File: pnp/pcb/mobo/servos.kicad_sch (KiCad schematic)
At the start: 2 parts, among them J15 SERVO1, J16 SERVO2

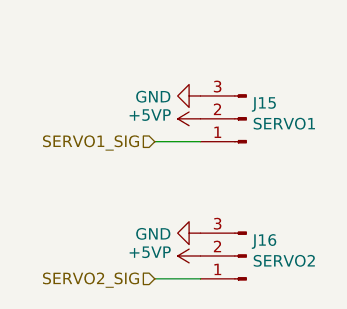
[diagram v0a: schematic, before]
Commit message: All sheets cleaned up
All symbols and their fields are now neatly organized.

All hierarchical pins are already imported,
except for the microcontroller sheet.
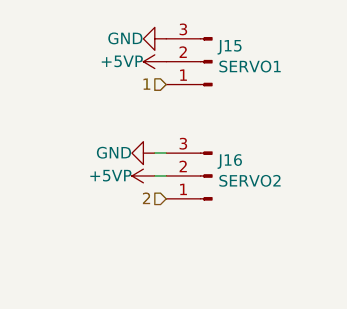
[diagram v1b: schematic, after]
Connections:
- net SERVO1_SIG renamed 1
- net SERVO2_SIG renamed 2
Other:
- moved on the sheet: J15, J16
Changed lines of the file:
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@@
 (kicad_sch (version 20211123) (generator eeschema)
   (paper "A4")
-  (wire (pts (xy 148.59 120.65) (xy 153.67 120.65))
+  (wire (pts (xy 148.59 106.68) (xy 149.86 106.68))
     (stroke (width 0) (type default) (color 0 0 0 0))
   )
-  (wire (pts (xy 148.59 105.41) (xy 153.67 105.41))
+  (wire (pts (xy 148.59 109.22) (xy 149.86 109.22))
     (stroke (width 0) (type default) (color 0 0 0 0))
   )
-  (hierarchical_label "SERVO1_SIG" (shape input) (at 148.59 105.41 180)
+  (hierarchical_label "1" (shape input) (at 149.86 99.06 180)
     (effects (font (size 1.27 1.27)) (justify right))
   )
-  (hierarchical_label "SERVO2_SIG" (shape input) (at 148.59 120.65 180)
+  (hierarchical_label "2" (shape input) (at 149.86 111.76 180)
     (effects (font (size 1.27 1.27)) (justify right))
   )
-  (symbol (lib_id "power:+5VP") (at 153.67 102.87 90) (unit 1)
+  (symbol (lib_id "power:+5VP") (at 149.86 96.52 90) (unit 1)
     (in_bom yes) (on_board yes)
-    (property "Reference" "#PWR0171" (id 0) (at 157.48 102.87 0)
+    (property "Reference" "#PWR0171" (id 0) (at 153.67 96.52 0)
       (effects (font (size 1.27 1.27)) hide)
     )
-    (property "Value" "+5VP" (id 1) (at 150.4188 102.489 90)
+    (property "Value" "+5VP" (id 1) (at 147.32 96.52 90)
       (effects (font (size 1.27 1.27)) (justify left))
     )
-    (property "Footprint" "" (id 2) (at 153.67 102.87 0)
+    (property "Footprint" "" (id 2) (at 149.86 96.52 0)
       (effects (font (size 1.27 1.27)) hide)
     )
-    (property "Datasheet" "" (id 3) (at 153.67 102.87 0)
+    (property "Datasheet" "" (id 3) (at 149.86 96.52 0)
       (effects (font (size 1.27 1.27)) hide)
     )
     (pin "1")
   )
-  (symbol (lib_id "power:GND") (at 153.67 100.33 270) (unit 1)
+  (symbol (lib_id "power:GND") (at 149.86 93.98 270) (unit 1)
     (in_bom yes) (on_board yes)
-    (property "Reference" "#PWR0170" (id 0) (at 147.32 100.33 0)
+    (property "Reference" "#PWR0170" (id 0) (at 143.51 93.98 0)
       (effects (font (size 1.27 1.27)) hide)
     )
-    (property "Value" "GND" (id 1) (at 150.4188 100.457 90)
+    (property "Value" "GND" (id 1) (at 147.32 93.98 90)
       (effects (font (size 1.27 1.27)) (justify right))
     )
-    (property "Footprint" "" (id 2) (at 153.67 100.33 0)
+    (property "Footprint" "" (id 2) (at 149.86 93.98 0)
       (effects (font (size 1.27 1.27)) hide)
     )
-    (property "Datasheet" "" (id 3) (at 153.67 100.33 0)
+    (property "Datasheet" "" (id 3) (at 149.86 93.98 0)
       (effects (font (size 1.27 1.27)) hide)
     )
     (pin "1")
   )
-  (symbol (lib_id "power:GND") (at 153.67 115.57 270) (unit 1)
+  (symbol (lib_id "power:GND") (at 148.59 106.68 270) (unit 1)
     (in_bom yes) (on_board yes)
-    (property "Reference" "#PWR0172" (id 0) (at 147.32 115.57 0)
+    (property "Reference" "#PWR0172" (id 0) (at 142.24 106.68 0)
       (effects (font (size 1.27 1.27)) hide)
     )
-    (property "Value" "GND" (id 1) (at 150.4188 115.697 90)
+    (property "Value" "GND" (id 1) (at 146.05 106.68 90)
       (effects (font (size 1.27 1.27)) (justify right))
     )
-    (property "Footprint" "" (id 2) (at 153.67 115.57 0)
+    (property "Footprint" "" (id 2) (at 148.59 106.68 0)
       (effects (font (size 1.27 1.27)) hide)
     )
-    (property "Datasheet" "" (id 3) (at 153.67 115.57 0)
+    (property "Datasheet" "" (id 3) (at 148.59 106.68 0)
       (effects (font (size 1.27 1.27)) hide)
     )
     (pin "1")
   )
-  (symbol (lib_id "power:+5VP") (at 153.67 118.11 90) (unit 1)
+  (symbol (lib_id "power:+5VP") (at 148.59 109.22 90) (unit 1)
     (in_bom yes) (on_board yes)
-    (property "Reference" "#PWR0173" (id 0) (at 157.48 118.11 0)
+    (property "Reference" "#PWR0173" (id 0) (at 152.4 109.22 0)
       (effects (font (size 1.27 1.27)) hide)
     )
-    (property "Value" "+5VP" (id 1) (at 150.4188 117.729 90)
+    (property "Value" "+5VP" (id 1) (at 146.05 109.22 90)
       (effects (font (size 1.27 1.27)) (justify left))
     )
-    (property "Footprint" "" (id 2) (at 153.67 118.11 0)
+    (property "Footprint" "" (id 2) (at 148.59 109.22 0)
       (effects (font (size 1.27 1.27)) hide)
     )
-    (property "Datasheet" "" (id 3) (at 153.67 118.11 0)
+    (property "Datasheet" "" (id 3) (at 148.59 109.22 0)
       (effects (font (size 1.27 1.27)) hide)
     )
     (pin "1")
   )
-  (symbol (lib_id "Connector:Conn_01x03_Male") (at 158.75 102.87 180) (unit 1)
+  (symbol (lib_id "Connector:Conn_01x03_Male") (at 154.94 96.52 180) (unit 1)
     (in_bom yes) (on_board yes)
-    (property "Reference" "J15" (id 0) (at 159.4612 101.1428 0)
+    (property "Reference" "J15" (id 0) (at 155.6512 94.7928 0)
       (effects (font (size 1.27 1.27)) (justify right))
     )
-    (property "Value" "SERVO1" (id 1) (at 159.4612 103.4542 0)
+    (property "Value" "SERVO1" (id 1) (at 155.6512 97.1042 0)
       (effects (font (size 1.27 1.27)) (justify right))
     )
-    (property "Footprint" "Connector_JST:JST_XH_B3B-XH-A_1x03_P2.50mm_Vertical" (id 2) (at 158.75 102.87 0)
+    (property "Footprint" "Connector_JST:JST_XH_B3B-XH-A_1x03_P2.50mm_Vertical" (id 2) (at 154.94 96.52 0)
       (effects (font (size 1.27 1.27)) hide)
     )
-    (property "Datasheet" "" (id 3) (at 158.75 102.87 0)
+    (property "Datasheet" "" (id 3) (at 154.94 96.52 0)
       (effects (font (size 1.27 1.27)) hide)
     )
-    (property "LCSC" "C2316" (id 4) (at 158.75 102.87 0)
+    (property "LCSC" "C2316" (id 4) (at 154.94 96.52 0)
       (effects (font (size 1.27 1.27)) hide)
     )
-    (property "JLCPCB" "C2316" (id 5) (at 158.75 102.87 0)
+    (property "JLCPCB" "C2316" (id 5) (at 154.94 96.52 0)
       (effects (font (size 1.27 1.27)) hide)
     )
-    (property "Digikey" "455-2248-ND" (id 6) (at 158.75 102.87 0)
+    (property "Digikey" "455-2248-ND" (id 6) (at 154.94 96.52 0)
       (effects (font (size 1.27 1.27)) hide)
     )
@@
     (pin "3")
   )
-  (symbol (lib_id "Connector:Conn_01x03_Male") (at 158.75 118.11 180) (unit 1)
+  (symbol (lib_id "Connector:Conn_01x03_Male") (at 154.94 109.22 180) (unit 1)
     (in_bom yes) (on_board yes)
-    (property "Reference" "J16" (id 0) (at 159.4612 116.3828 0)
+    (property "Reference" "J16" (id 0) (at 155.6512 107.4928 0)
       (effects (font (size 1.27 1.27)) (justify right))
     )
-    (property "Value" "SERVO2" (id 1) (at 159.4612 118.6942 0)
+    (property "Value" "SERVO2" (id 1) (at 155.6512 109.8042 0)
       (effects (font (size 1.27 1.27)) (justify right))
     )
-    (property "Footprint" "Connector_JST:JST_XH_B3B-XH-A_1x03_P2.50mm_Vertical" (id 2) (at 158.75 118.11 0)
+    (property "Footprint" "Connector_JST:JST_XH_B3B-XH-A_1x03_P2.50mm_Vertical" (id 2) (at 154.94 109.22 0)
       (effects (font (size 1.27 1.27)) hide)
     )
-    (property "Datasheet" "" (id 3) (at 158.75 118.11 0)
+    (property "Datasheet" "" (id 3) (at 154.94 109.22 0)
       (effects (font (size 1.27 1.27)) hide)
     )
-    (property "LCSC" "C2316" (id 4) (at 158.75 118.11 0)
+    (property "LCSC" "C2316" (id 4) (at 154.94 109.22 0)
       (effects (font (size 1.27 1.27)) hide)
     )
-    (property "JLCPCB" "C2316" (id 5) (at 158.75 118.11 0)
+    (property "JLCPCB" "C2316" (id 5) (at 154.94 109.22 0)
       (effects (font (size 1.27 1.27)) hide)
     )
-    (property "Digikey" "455-2248-ND" (id 6) (at 158.75 118.11 0)
+    (property "Digikey" "455-2248-ND" (id 6) (at 154.94 109.22 0)
       (effects (font (size 1.27 1.27)) hide)
     )
